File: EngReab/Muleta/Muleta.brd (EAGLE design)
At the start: 53.3 x 56.8 mm, 16 parts, among them IC1 REF01Z, IC2 INA110KP, IC3 LF356N, J1 RJ11-6X

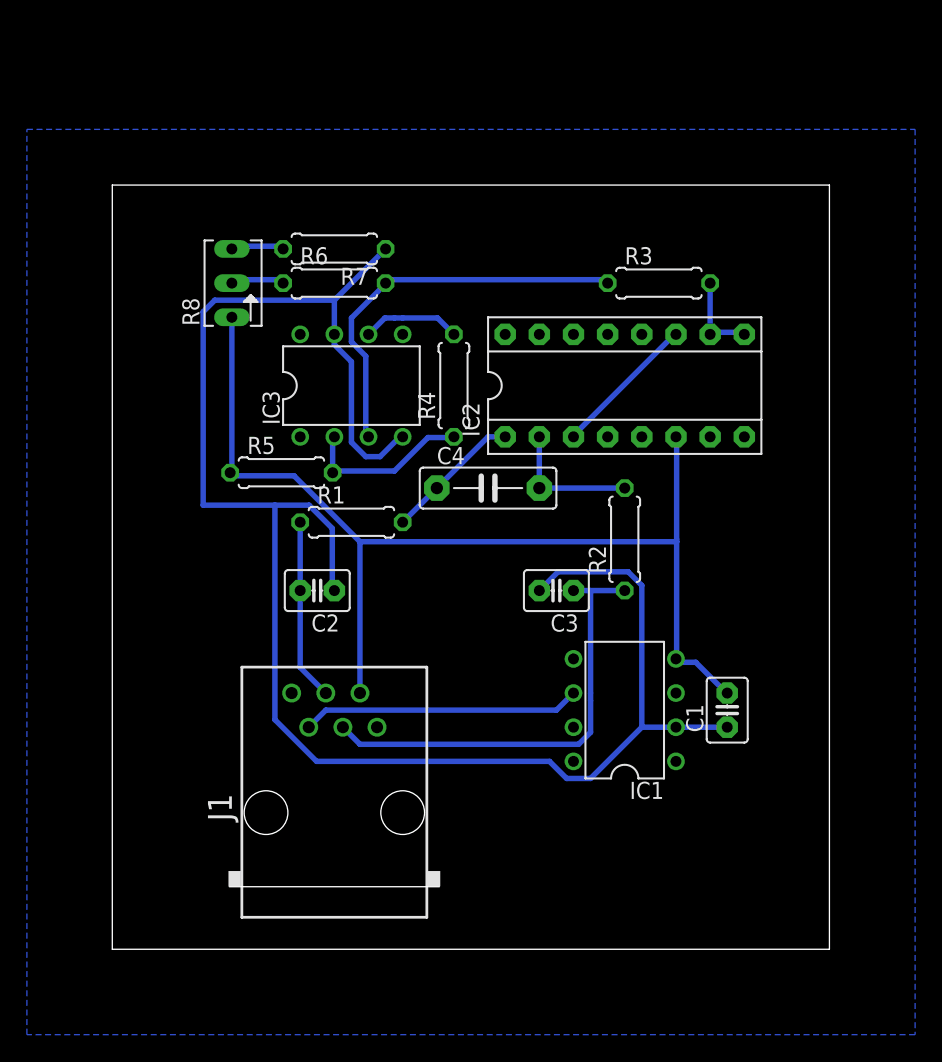
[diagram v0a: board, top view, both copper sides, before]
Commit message: Saida Analog A5?
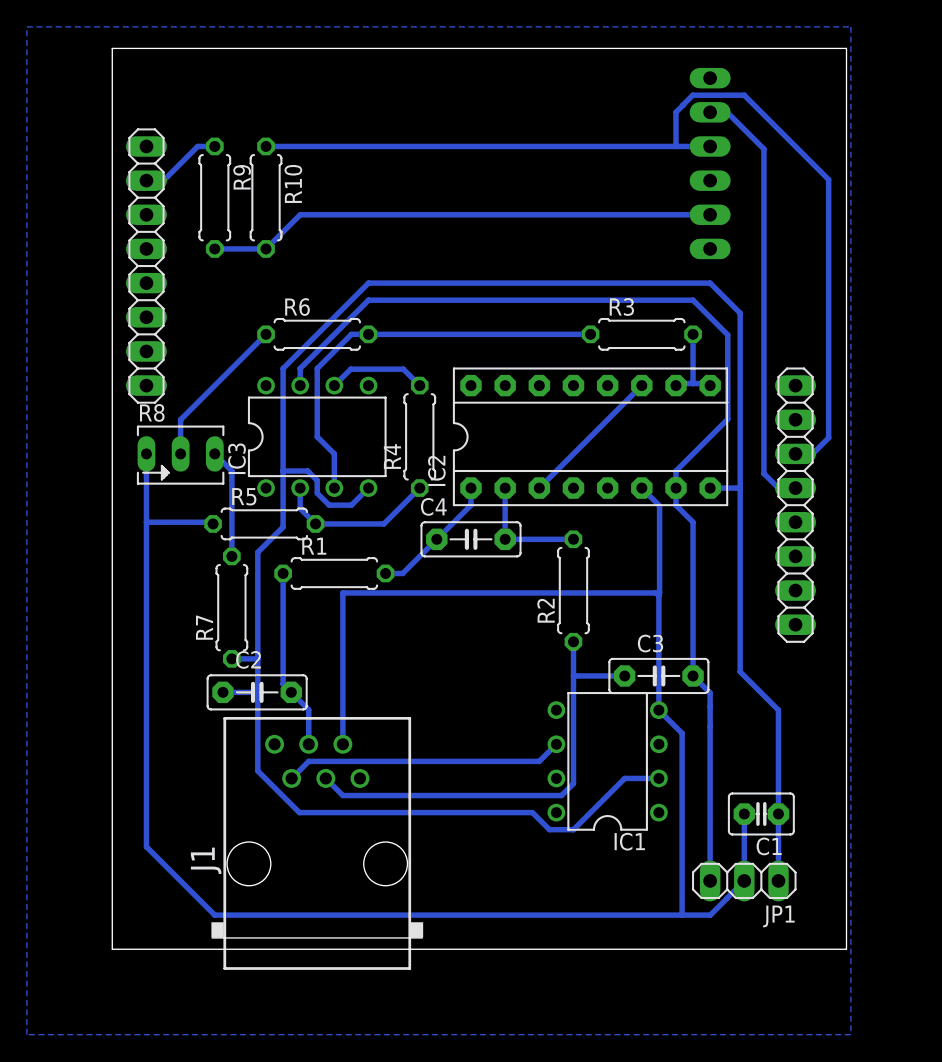
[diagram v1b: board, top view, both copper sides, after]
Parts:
- added HC05: (no value), pinhead:1X06/90
- added IOL1, POWER1: (no value), pinhead:1X08
- added JP1: (no value), pinhead:1X03
- added R10: 2k2R, resistor:0207/7
- added R9: 1k5R, resistor:0207/7
- C2, C3: device capacitor-wima:C2.5-3 -> capacitor-wima:C5B2.5
- C4: device capacitor-wima:C7.5B3 -> capacitor-wima:C5B2.5
- moved R7 27.7 mm to (8.89, 25.4), turned to 90 degrees
- moved R8 13.3 mm to (5.08, 36.8), turned to 0 degrees
- moved C3 9.92 mm to (40.6, 20.3), turned to 0 degrees
- moved C2 8.79 mm to (10.8, 19.1), turned to 0 degrees
- moved C1 8.13 mm to (48.3, 10.1), turned to 180 degrees
- moved R2 5.39 mm to (34.3, 26.7)
- moved IC3 4.58 mm to (15.2, 38.1)
- moved IC2 4.58 mm to (35.6, 38.1)
- moved R4 4.58 mm to (22.9, 38.1)
- moved R3 4.02 mm to (39.4, 45.7)
- moved R6 4.02 mm to (15.2, 45.7)
- moved IC1 4.02 mm to (36.8, 14.0)
- moved J1 4.02 mm to (15.2, 6.35)
- moved C4 4.02 mm to (26.7, 30.5)
- moved R1 4.02 mm to (16.5, 27.9)
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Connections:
- removed net +VCC: IC2.8
- removed net -VCC: IC2.7
- removed net VCC: C1.1, C2.1, C3.2, IC1.2, IC3.4, IC3.7, R7.1
- new net +15V: C1.1, C2.1, IC1.2, IC2.8, IC3.4, JP1.1, R7.1
- new net -15V: C3.2, IC2.7, IC3.7, JP1.3
- new net ARDUINO_5V: HC05.2, POWER1.5
- new net ARDUINO_DIG: IOL1.2, R9.1
- new net ARDUINO_GND: HC05.3, POWER1.6, R10.1
- new net N$15: HC05.5, R10.2, R9.2
- net GND: now also JP1.2
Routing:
- net +15V: track 0.00 -> 160.1 mm
- net VCC: track 133.0 -> 0.00 mm
- net -15V: track 0.00 -> 79.5 mm
- net GND: track 79.7 -> 154.7 mm
- net ARDUINO_GND: track 0.00 -> 72.2 mm
- net N$15: track 0.00 -> 37.9 mm
- net ARDUINO_5V: track 0.00 -> 32.1 mm
- net N$1: track 4.17 -> 11.5 mm
- net ARDUINO_DIG: track 0.00 -> 6.13 mm
- net N$2: track 4.08 -> 8.15 mm
- net N$6: track 10.2 -> 8.89 mm
- net N$14: track 29.7 -> 30.8 mm
- net N$13: track 12.8 -> 12.2 mm
- net N$7: track 10.3 -> 9.72 mm
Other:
- board size 53.3 x 56.8 mm -> 54.6 x 67 mm
- board text added: "D:/SmartProjects/Snc/a4_bn_logo2.bmp"
